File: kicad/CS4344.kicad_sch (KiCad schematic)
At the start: 0 parts

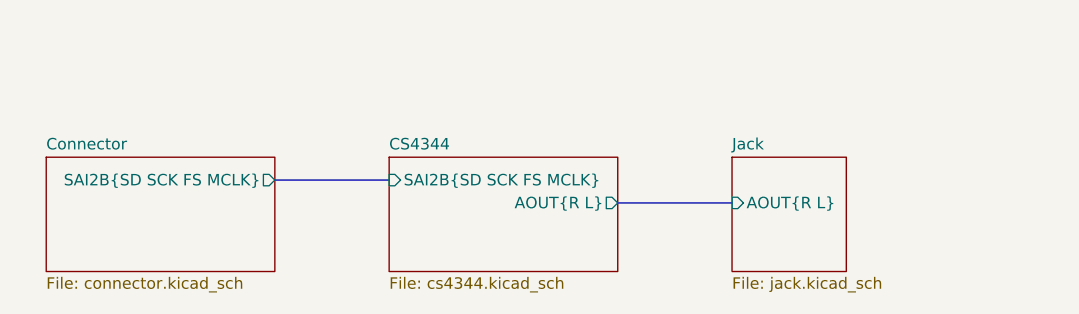
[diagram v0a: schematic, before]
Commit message: journal and readme
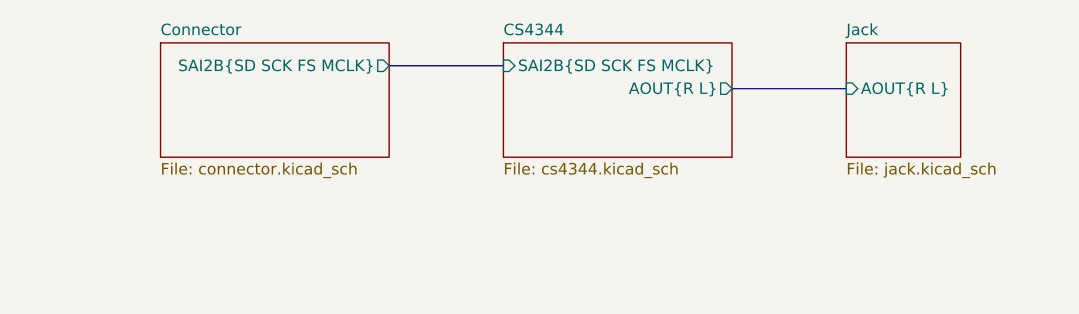
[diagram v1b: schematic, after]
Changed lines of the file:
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@@
 	(bus
 		(pts
-			(xy 38.1 40.64) (xy 50.8 40.64)
+			(xy 50.8 27.94) (xy 63.5 27.94)
 		)
 		(stroke
@@
 	(bus
 		(pts
-			(xy 76.2 43.18) (xy 88.9 43.18)
+			(xy 88.9 30.48) (xy 101.6 30.48)
 		)
 		(stroke
@@
 	)
 	(sheet
-		(at 50.8 38.1)
+		(at 63.5 25.4)
 		(size 25.4 12.7)
 		(exclude_from_sim no)
@@
 		)
 		(property "Sheetname" "CS4344"
-			(at 50.8 37.3884 0)
+			(at 63.5 24.6884 0)
 			(show_name no)
 			(do_not_autoplace no)
@@
 		)
 		(property "Sheetfile" "cs4344.kicad_sch"
-			(at 50.8 51.3846 0)
+			(at 63.5 38.6846 0)
 			(show_name no)
 			(do_not_autoplace no)
@@
 		)
 		(pin "AOUT{R L}" output
-			(at 76.2 43.18 0)
+			(at 88.9 30.48 0)
 			(effects
 				(font
@@
 		)
 		(pin "SAI2B{SD SCK FS MCLK}" input
-			(at 50.8 40.64 180)
+			(at 63.5 27.94 180)
 			(effects
 				(font
@@
 	)
 	(sheet
-		(at 12.7 38.1)
+		(at 25.4 25.4)
 		(size 25.4 12.7)
 		(exclude_from_sim no)
@@
 		)
 		(property "Sheetname" "Connector"
-			(at 12.7 37.3884 0)
+			(at 25.4 24.6884 0)
 			(show_name no)
 			(do_not_autoplace no)
@@
 		)
 		(property "Sheetfile" "connector.kicad_sch"
-			(at 12.7 51.3846 0)
+			(at 25.4 38.6846 0)
 			(show_name no)
 			(do_not_autoplace no)
@@
 		)
 		(pin "SAI2B{SD SCK FS MCLK}" output
-			(at 38.1 40.64 0)
+			(at 50.8 27.94 0)
 			(effects
 				(font
@@
 	)
 	(sheet
-		(at 88.9 38.1)
+		(at 101.6 25.4)
 		(size 12.7 12.7)
 		(exclude_from_sim no)
@@
 		)
 		(property "Sheetname" "Jack"
-			(at 88.9 37.3884 0)
+			(at 101.6 24.6884 0)
 			(show_name no)
 			(do_not_autoplace no)
@@
 		)
 		(property "Sheetfile" "jack.kicad_sch"
-			(at 88.9 51.3846 0)
+			(at 101.6 38.6846 0)
 			(show_name no)
 			(do_not_autoplace no)
@@
 		)
 		(pin "AOUT{R L}" input
-			(at 88.9 43.18 180)
+			(at 101.6 30.48 180)
 			(effects
 				(font
